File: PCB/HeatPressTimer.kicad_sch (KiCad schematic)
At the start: 6 parts, among them J1 2" SPI ST7789VW Display, J2 Piezo, SW1 Switch, SW2 Switch, SW3 Vertical Limit Switch, U1 XIAO-ESP32-C6

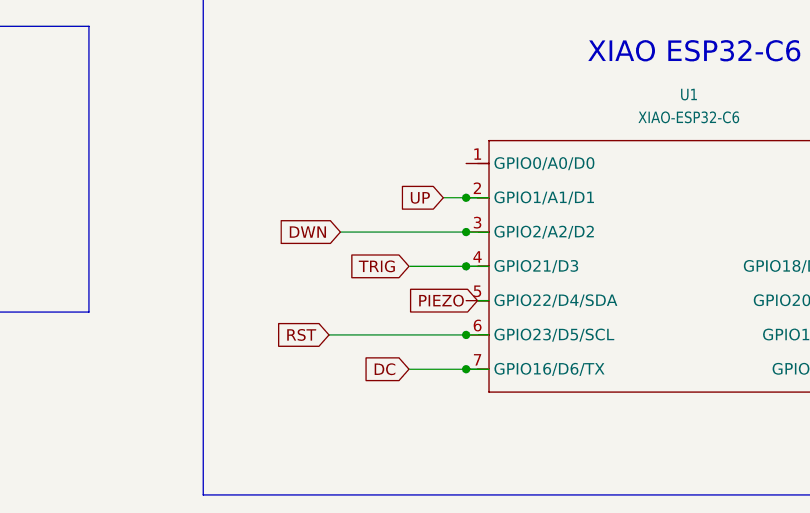
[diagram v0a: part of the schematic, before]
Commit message: new PCB files
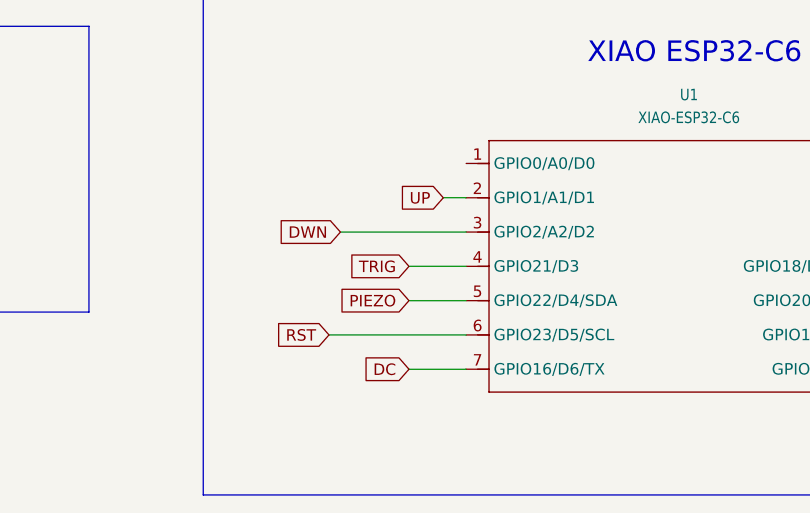
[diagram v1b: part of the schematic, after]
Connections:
- net PIEZO: now also U1.5 (GPIO22/D4/SDA)
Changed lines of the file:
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@@
 	(generator_version "8.0")
 	(paper "A4")
-	(junction
-		(at 121.92 127)
-		(diameter 0)
-		(color 0 0 0 0)
-	)
-	(junction
-		(at 121.92 146.05)
-		(diameter 0)
-		(color 0 0 0 0)
-	)
-	(junction
-		(at 121.92 130.81)
-		(diameter 0)
-		(color 0 0 0 0)
-	)
-	(junction
-		(at 121.92 142.24)
-		(diameter 0)
-		(color 0 0 0 0)
-	)
-	(junction
-		(at 121.92 134.62)
-		(diameter 0)
-		(color 0 0 0 0)
-	)
 	(wire
 		(pts
@@
 	(wire
 		(pts
-			(xy 123.19 138.43) (xy 124.46 138.43)
-		)
-		(stroke
-			(width 0)
-			(type default)
-		)
-	)
-	(wire
-		(pts
 			(xy 109.22 88.9) (xy 114.3 88.9)
 		)
@@
 	(wire
 		(pts
+			(xy 115.57 138.43) (xy 121.92 138.43)
+		)
+		(stroke
+			(width 0)
+			(type default)
+		)
+	)
+	(wire
+		(pts
 			(xy 154.94 88.9) (xy 163.83 88.9)
 		)
@@
 	(wire
 		(pts
-			(xy 121.92 142.24) (xy 124.46 142.24)
-		)
-		(stroke
-			(width 0)
-			(type default)
-		)
-	)
-	(wire
-		(pts
 			(xy 57.15 129.54) (xy 62.23 129.54)
 		)
@@
 	(wire
 		(pts
-			(xy 121.92 146.05) (xy 124.46 146.05)
-		)
-		(stroke
-			(width 0)
-			(type default)
-		)
-	)
-	(wire
-		(pts
-			(xy 121.92 130.81) (xy 124.46 130.81)
-		)
-		(stroke
-			(width 0)
-			(type default)
-		)
-	)
-	(wire
-		(pts
 			(xy 115.57 146.05) (xy 121.92 146.05)
 		)
@@
 	(wire
 		(pts
-			(xy 121.92 127) (xy 124.46 127)
-		)
-		(stroke
-			(width 0)
-			(type default)
-		)
-	)
-	(wire
-		(pts
 			(xy 171.45 146.05) (xy 189.23 146.05)
 		)
@@
 		(pts
 			(xy 107.95 130.81) (xy 121.92 130.81)
-		)
-		(stroke
-			(width 0)
-			(type default)
-		)
-	)
-	(wire
-		(pts
-			(xy 121.92 134.62) (xy 124.46 134.62)
 		)
 		(stroke
@@
 	(global_label "PIEZO"
 		(shape input)
-		(at 123.19 138.43 180)
+		(at 115.57 138.43 180)
 		(fields_autoplaced yes)
 		(effects
@@
 		)
 		(property "Intersheetrefs" "${INTERSHEET_REFS}"
-			(at 114.641 138.43 0)
-			(effects
-				(font
+			(at 107.021 138.43 0)
+			(effects
+				(font
